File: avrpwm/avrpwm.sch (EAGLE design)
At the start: 54 parts, among them IC1 7805TV, IC2 AT90S2313P, Q1 BC337-40, Q10 BC337-40, Q11 BC337-40, Q12 BC337-40, Q13 BC337-40, Q2 BC337-40, Q3 BC337-40, Q4 BC337-40, Q5 BC337-40, Q6 BC337-40, Q7 BC337-40, Q8 BC337-40, Q9 BC337-40

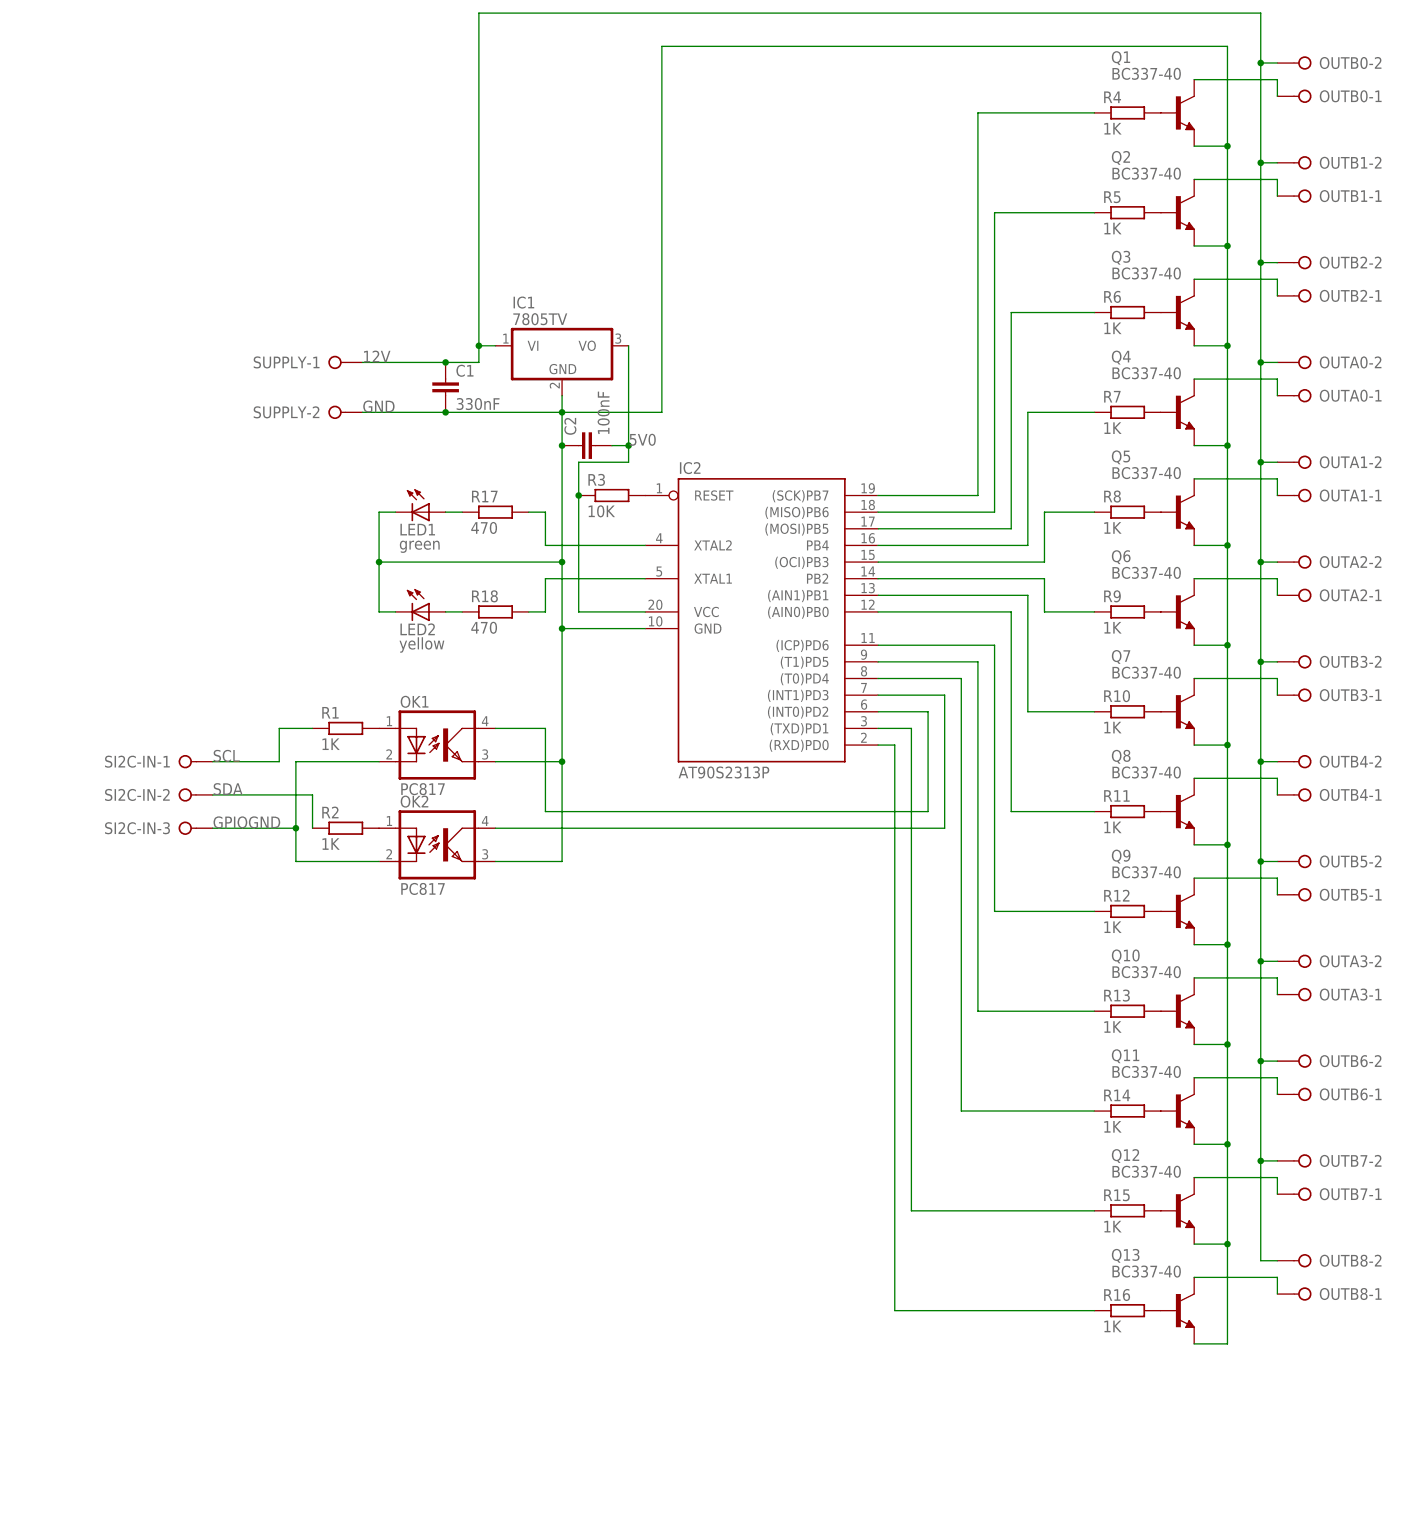
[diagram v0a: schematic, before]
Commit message: moar eagle
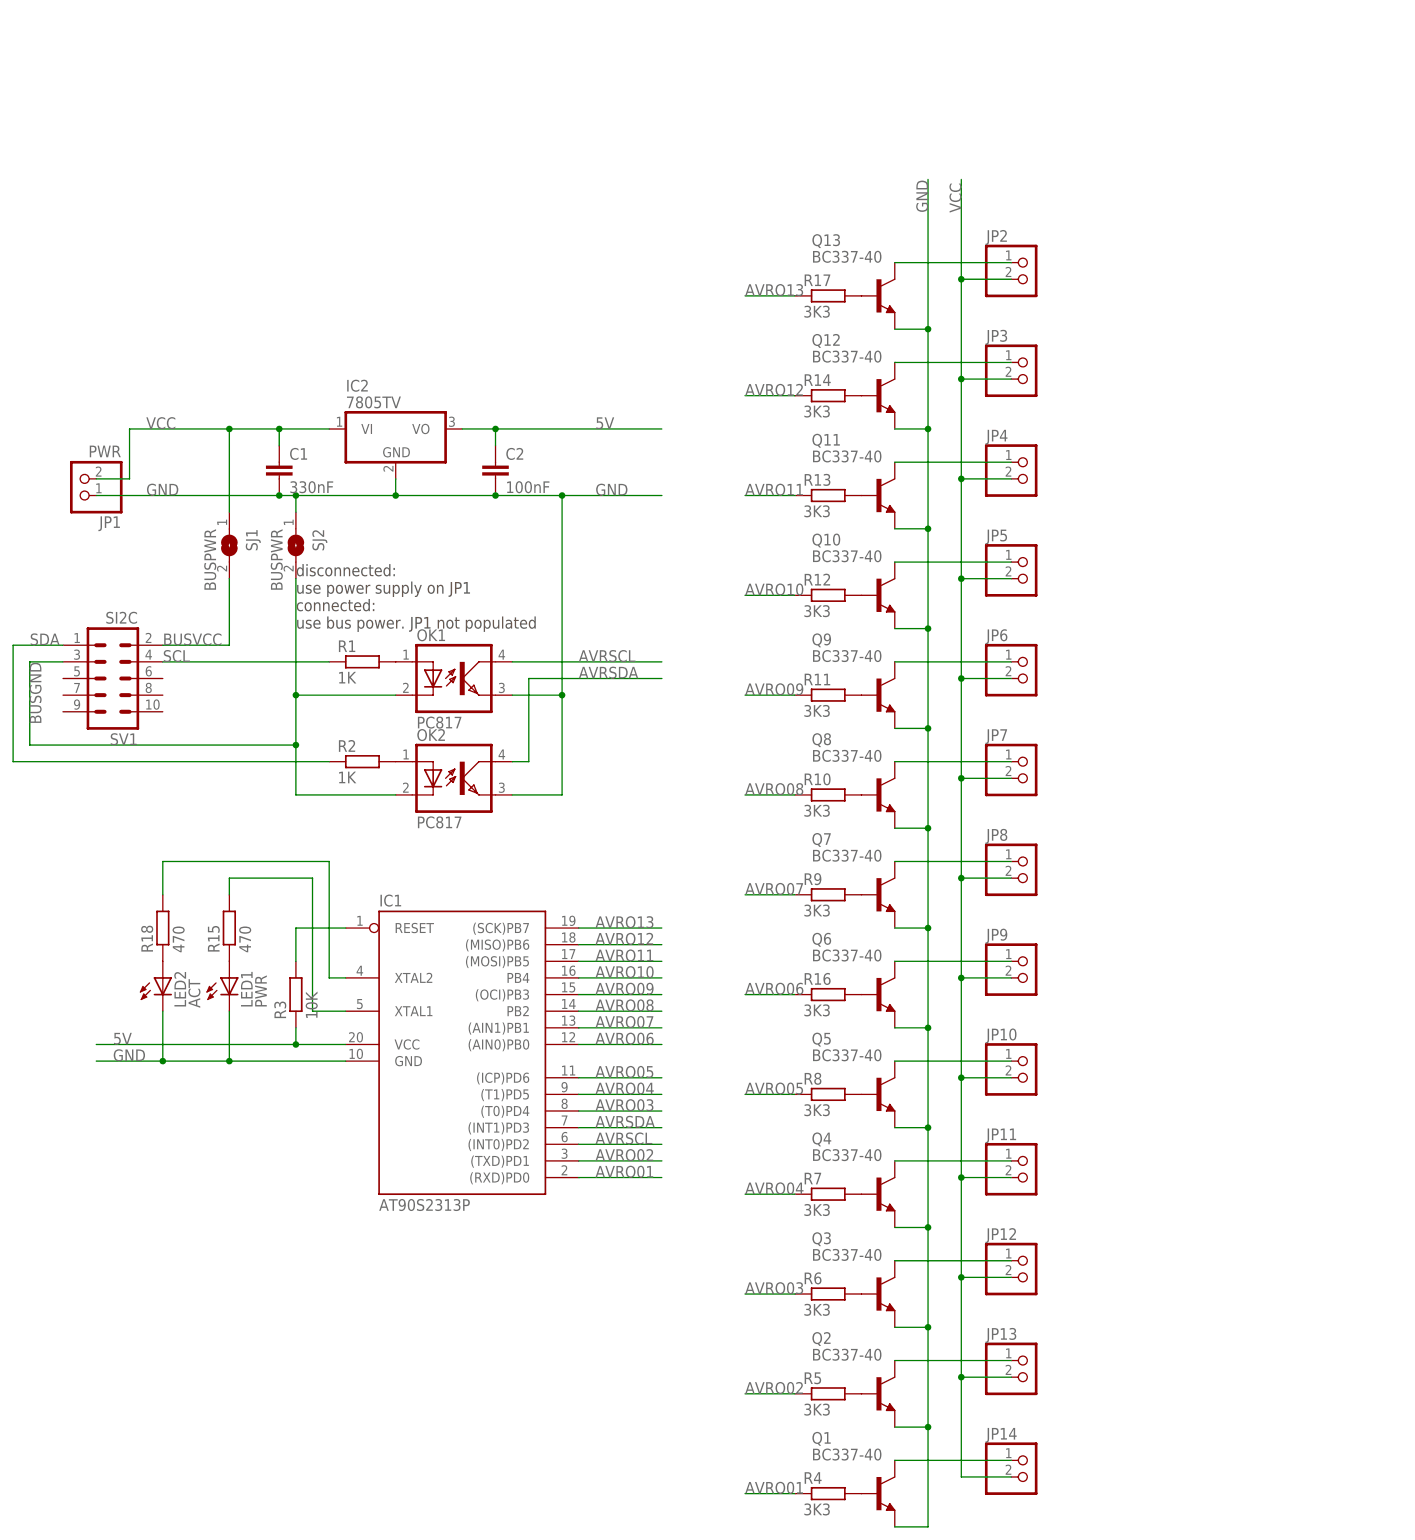
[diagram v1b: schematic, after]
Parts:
- removed OUTA0, OUTA1, OUTA2, OUTA3, OUTB0, OUTB1, OUTB2, OUTB3, OUTB4, OUTB5, OUTB6, OUTB7, OUTB8, SUPPLY: (no value), con-wago-508:W237-02P
- removed SI2C-IN: (no value), con-wago-508:W237-3E
- added JP1: PWR, pinhead:PINHD-1X2
- added JP10, JP11, JP12, JP13, JP14, JP2, JP3, JP4, JP5, JP6, JP7, JP8, JP9: (no value), pinhead:PINHD-1X2
- added SJ1, SJ2: BUSPWR, jumper:SJ
- added SV1: SI2C, con-harting-ml:ML10
- IC1: value 7805TV -> AT90S2313P; device linear:7805TV -> atmel:AT90S2313P
- IC2: value AT90S2313P -> 7805TV; device atmel:AT90S2313P -> linear:7805TV
- LED1: value green -> PWR
- LED2: value yellow -> ACT
- R10, R11, R12, R13, R14, R16, R4, R5, R6, R7, R8, R9: value 1K -> 3K3
- R15: value 1K -> 470
- R17: value 470 -> 3K3
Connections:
- removed net 12V: C1.1, IC1.VI, OUTA0-2.KL, OUTA1-2.KL, OUTA2-2.KL, OUTA3-2.KL, OUTB0-2.KL, OUTB1-2.KL, OUTB2-2.KL, OUTB3-2.KL, OUTB4-2.KL, OUTB5-2.KL, OUTB6-2.KL, OUTB7-2.KL, OUTB8-2.KL, SUPPLY-1.KL
- removed net 5V0: C2.2, IC1.VO, IC2.VCC, R3.1
- removed net GPIOGND: OK1.C, OK2.C, SI2C-IN-3.KL
- removed net N$11 (its old number): Q12.B, R15.2
- removed net N$12 (its old number): Q13.B, R16.2
- removed net N$13 (its old number): IC2.(T1)PD5, R13.1
- removed net N$14 (its old number): Q9.B, R12.2
- removed net N$2: IC2.RESET, R3.2
- removed net N$24: IC2.(RXD)PD0, R16.1
- removed net N$25: OUTB7-1.KL, Q12.C
- removed net N$26: OUTA3-1.KL, Q10.C
- removed net N$27: IC2.(ICP)PD6, R12.1
- removed net N$28: IC2.(AIN0)PB0, R11.1
- removed net N$29: IC2.(AIN1)PB1, R10.1
- removed net N$30: IC2.PB2, R9.1
- removed net N$31: IC2.(OCI)PB3, R8.1
- removed net N$32: IC2.PB4, R7.1
- removed net N$34: IC2.(MISO)PB6, R5.1
- removed net N$35: OUTB6-1.KL, Q11.C
- removed net N$36: OUTB8-1.KL, Q13.C
- removed net N$38: IC2.XTAL1, R18.2
- removed net N$48: OUTB1-1.KL, Q2.C
- removed net N$8 (its old number): IC2.(INT1)PD3, OK2.COL
- removed net N$9 (its old number): Q11.B, R14.2
- new net 5V: C2.1, IC1.VCC, IC2.VO, R3.1
- new net AVRO01: IC1.(RXD)PD0, R4.1
- new net AVRO02: IC1.(TXD)PD1, R5.1
- new net AVRO03: IC1.(T0)PD4, R6.1
- new net AVRO04: IC1.(T1)PD5, R7.1
- new net AVRO05: IC1.(ICP)PD6, R8.1
- new net AVRO06: IC1.(AIN0)PB0, R16.1
- new net AVRO07: IC1.(AIN1)PB1, R9.1
- new net AVRO08: IC1.PB2, R10.1
- new net AVRO09: IC1.(OCI)PB3, R11.1
- new net AVRO10: IC1.PB4, R12.1
- new net AVRO11: IC1.(MOSI)PB5, R13.1
- new net AVRO12: IC1.(MISO)PB6, R14.1
- new net AVRO13: IC1.(SCK)PB7, R17.1
- new net AVRSCL: IC1.(INT0)PD2, OK1.COL
- new net AVRSDA: IC1.(INT1)PD3, OK2.COL
- new net BUSGND: OK1.C, OK2.C, SJ2.2, SV1.3
- new net BUSVCC: SJ1.2, SV1.2
- new net N$17: Q9.B, R11.2
- new net N$18: Q10.B, R12.2
- new net N$19: Q11.B, R13.2
- new net N$20: Q12.B, R14.2
- new net N$39: JP12.1, Q3.C
- new net N$5: Q13.B, R17.2
- new net VCC: C1.1, IC2.VI, JP1.2, JP10.2, JP11.2, JP12.2, JP13.2, JP14.2, JP2.2, JP3.2, JP4.2, JP5.2, JP6.2, JP7.2, JP8.2, JP9.2, SJ1.1
- net GND: now also C2.2, JP1.1, SJ2.1; no longer C2.1, SUPPLY-2.KL
- net N$10: now also LED1.A, R15.1; no longer IC2.(INT0)PD2, OK1.COL
- net N$15: now also R9.2; no longer R10.2
- net N$16: now also Q8.B, R10.2; no longer Q6.B, R9.2
- net N$21: now also IC1.XTAL2, R18.2; no longer IC2.(T0)PD4, R14.1
- net N$22: now also Q6.B, R16.2; no longer Q8.B, R11.2
- net N$23: now also JP3.1, Q12.C; no longer IC2.(TXD)PD1, R15.1
- net N$3: now also IC1.RESET, R3.2; no longer Q10.B, R13.2
- net N$33: now also IC1.XTAL1, R15.2; no longer IC2.(MOSI)PB5, R6.1
- net N$37: now also JP14.1, Q1.C; no longer IC2.XTAL2, R17.2
- net N$40: now also JP11.1, Q4.C; no longer LED1.A, R17.1
- net N$41: now also JP10.1, Q5.C; no longer OUTB5-1.KL, Q9.C
- net N$42: now also JP9.1, Q6.C; no longer OUTB4-1.KL, Q8.C
- net N$43: now also JP8.1; no longer OUTB3-1.KL
- net N$44: now also JP7.1, Q8.C; no longer OUTA2-1.KL, Q6.C
- net N$45: now also JP6.1, Q9.C; no longer OUTA1-1.KL, Q5.C
- net N$46: now also JP5.1, Q10.C; no longer OUTA0-1.KL, Q4.C
- net N$47: now also JP4.1, Q11.C; no longer OUTB2-1.KL, Q3.C
- net N$6: now also JP13.1, Q2.C; no longer OUTB0-1.KL, Q1.C
- net N$7: now also JP2.1, Q13.C; no longer IC2.(SCK)PB7, R4.1
- net SCL: now also SV1.4; no longer SI2C-IN-1.KL
- net SDA: now also SV1.1; no longer SI2C-IN-2.KL
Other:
- note added: "disconnected: use power supply on JP1 connected: use bus power. JP1 not populated"
- moved on the sheet: C1, C2, LED1, LED2, OK1, OK2, Q1, Q10, Q11, Q12, Q13, Q2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
